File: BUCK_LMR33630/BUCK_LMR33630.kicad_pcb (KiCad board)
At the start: 2 copper layers, 9 parts, among them U1 LMR33630ADDA

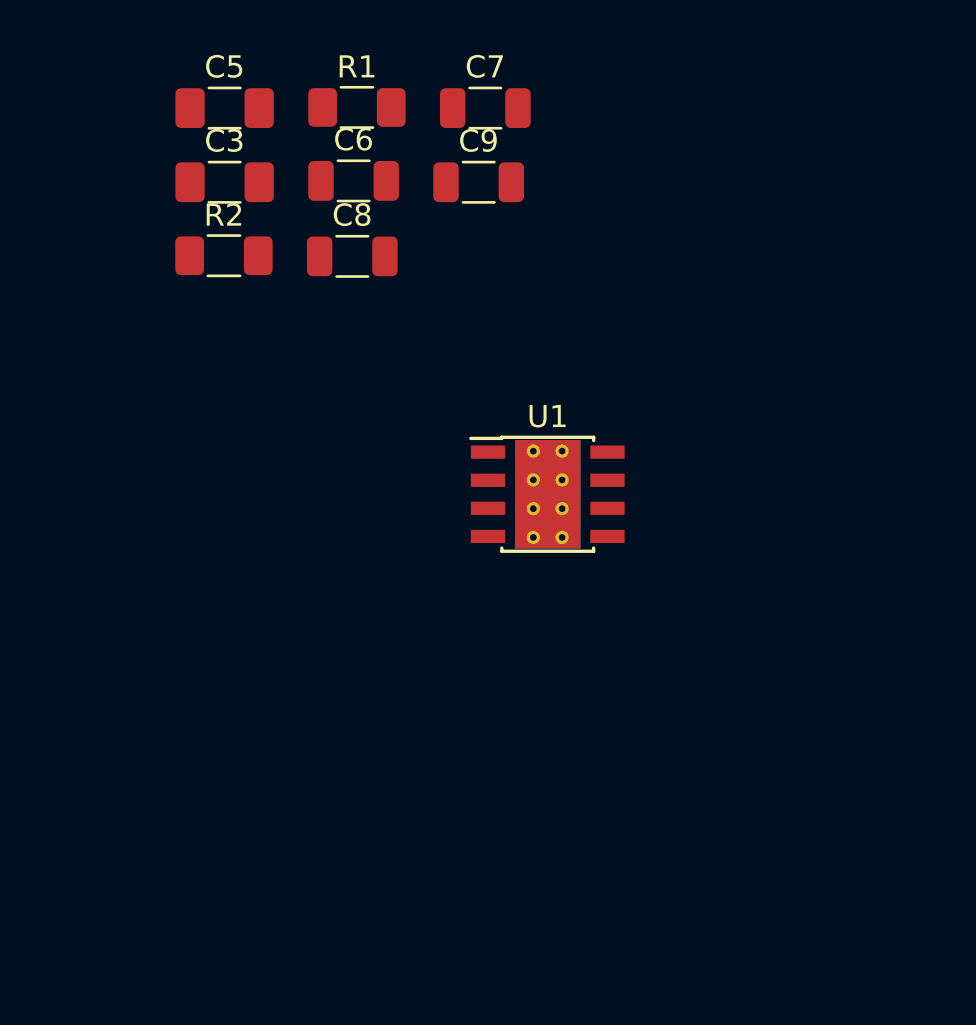
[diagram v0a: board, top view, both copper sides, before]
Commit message: Update doc
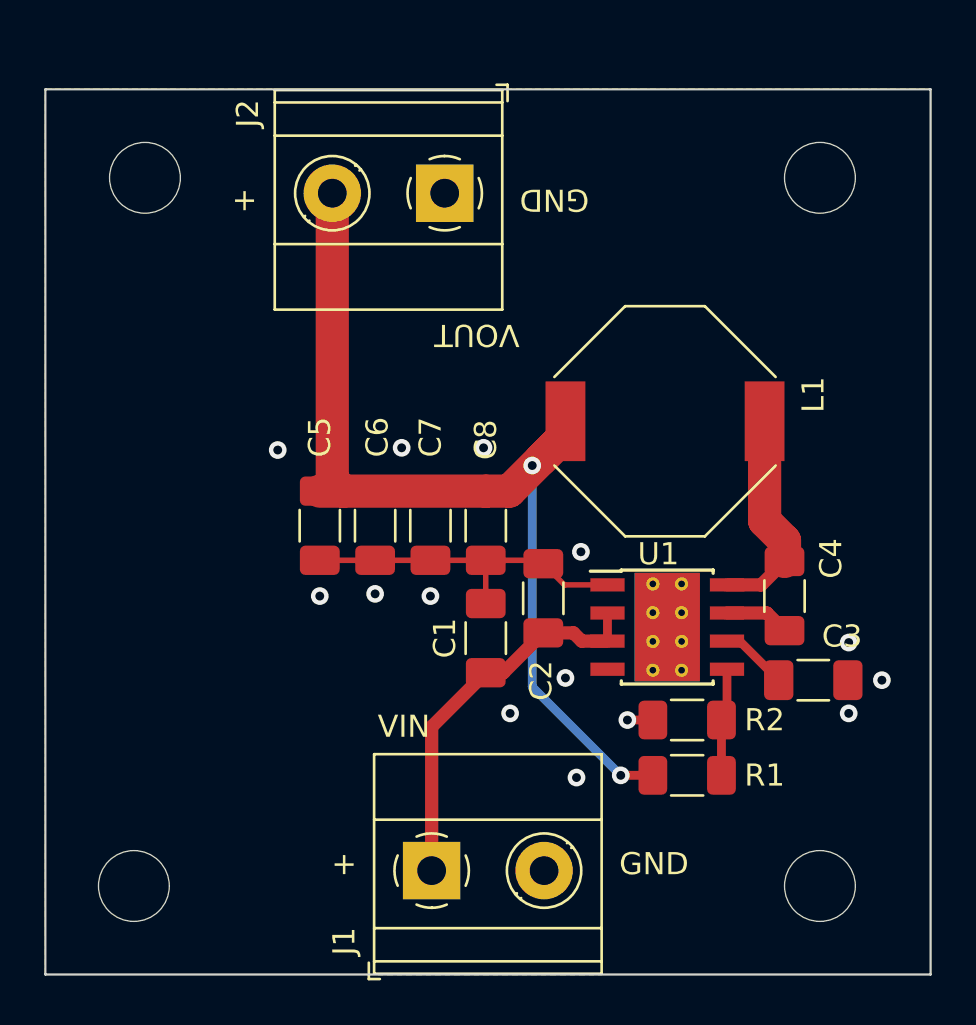
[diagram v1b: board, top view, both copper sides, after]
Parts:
- removed C9: 22uF, Capacitor_SMD:C_1206_3216Metric
- added C1: 10uF, Capacitor_SMD:C_1206_3216Metric_Pad1.33x1.80mm_HandSolder, F.Cu at (119.9, 84.8)
- added C2: 220nF, Capacitor_SMD:C_1206_3216Metric_Pad1.33x1.80mm_HandSolder, F.Cu at (122.5, 83.0)
- added C4: 100nF, Capacitor_SMD:C_1206_3216Metric_Pad1.33x1.80mm_HandSolder, F.Cu at (133.4, 82.9)
- added H1: MountingHole, MountingHole:MountingHole_3.2mm_M3, F.Cu at (104.0, 96.0)
- added H2: MountingHole, MountingHole:MountingHole_3.2mm_M3, F.Cu at (135.0, 96.0)
- added H3: MountingHole, MountingHole:MountingHole_3.2mm_M3, F.Cu at (104.5, 64.0)
- added H4: MountingHole, MountingHole:MountingHole_3.2mm_M3, F.Cu at (135.0, 64.0)
- added J1: Conn_01x02, TerminalBlock_Phoenix:TerminalBlock_Phoenix_MKDS-1,5-2-5.08_1x02_P5.08mm_Horizontal, F.Cu at (117.5, 95.3)
- added J2: Conn_01x02, TerminalBlock_Phoenix:TerminalBlock_Phoenix_MKDS-1,5-2-5.08_1x02_P5.08mm_Horizontal, F.Cu at (118.0, 64.7)
- added L1: 6.8uH, 14mΩ, Inductor_SMD:L_Bourns-SRU1028_10.0x10.0mm, F.Cu at (128.0, 75.0)
- C6, C7, C8: footprint Capacitor_SMD:C_1206_3216Metric -> Capacitor_SMD:C_1206_3216Metric_Pad1.33x1.80mm_HandSolder
- moved C3 34.8 mm to (134.7, 86.7)
- moved R1 33.7 mm to (129.0, 91.0)
- moved R2 29.6 mm to (129.0, 88.5), turned to 180 degrees
- moved C5 19.4 mm to (112.4, 79.7), turned to -90 degrees
- moved C7 19.0 mm to (117.4, 79.7), turned to -90 degrees
- moved C6 15.6 mm to (114.9, 79.7), turned to -90 degrees
- moved C8 13.6 mm to (119.9, 79.7), turned to -90 degrees
- moved U1 8.07 mm to (128.1, 84.3)
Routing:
- net VOUT: track 0.00 -> 45.1 mm, vias 0 -> 2
- net VIN: track 0.00 -> 17.6 mm
- net GND: track 0.00 -> 16.6 mm, vias 0 -> 14
- net Net-(C4-Pad1): track 0.00 -> 9.75 mm
- net Net-(R1-Pad2): track 0.00 -> 4.05 mm
- net Net-(C3-Pad1): track 0.00 -> 3.07 mm
- net Net-(C4-Pad2): track 0.00 -> 2.93 mm
- added copper zone on B.Cu, net GND
- added copper zone on F.Cu, net GND
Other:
- board outline added: 40 x 40 mm
- board text added: "+"
- board text added: "3.8V - 36V"
- board text added: "CERN-OHL-P v2"
- board text added: "GITHUB.COM/ZERBERROS"
- board text added: "GND"
- board text added: "LMR33630 BUCK REG."
- board text added: "VIN"
- board text added: "VOUT"
